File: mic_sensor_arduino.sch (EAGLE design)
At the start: 19 parts, among them U1 LM393DR, U2 LM393DR

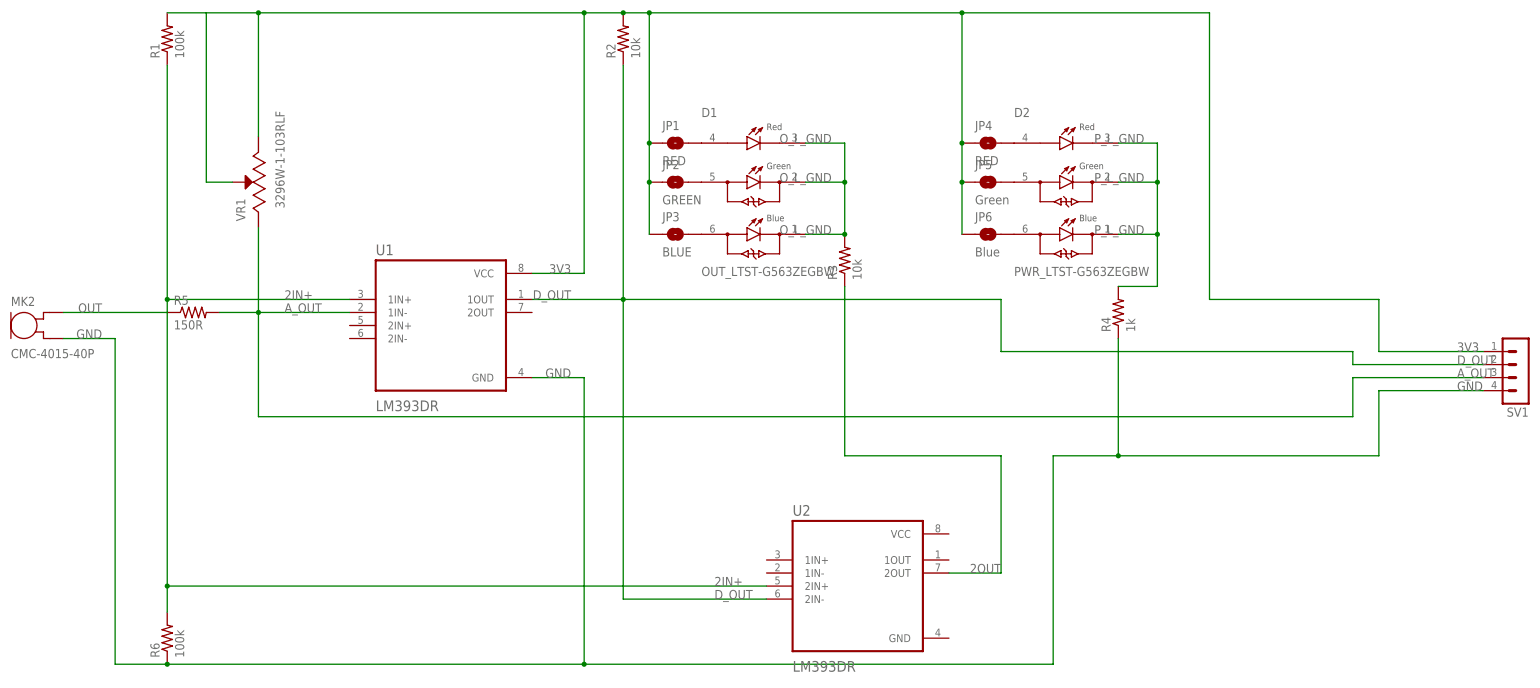
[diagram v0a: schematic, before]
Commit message: update resources
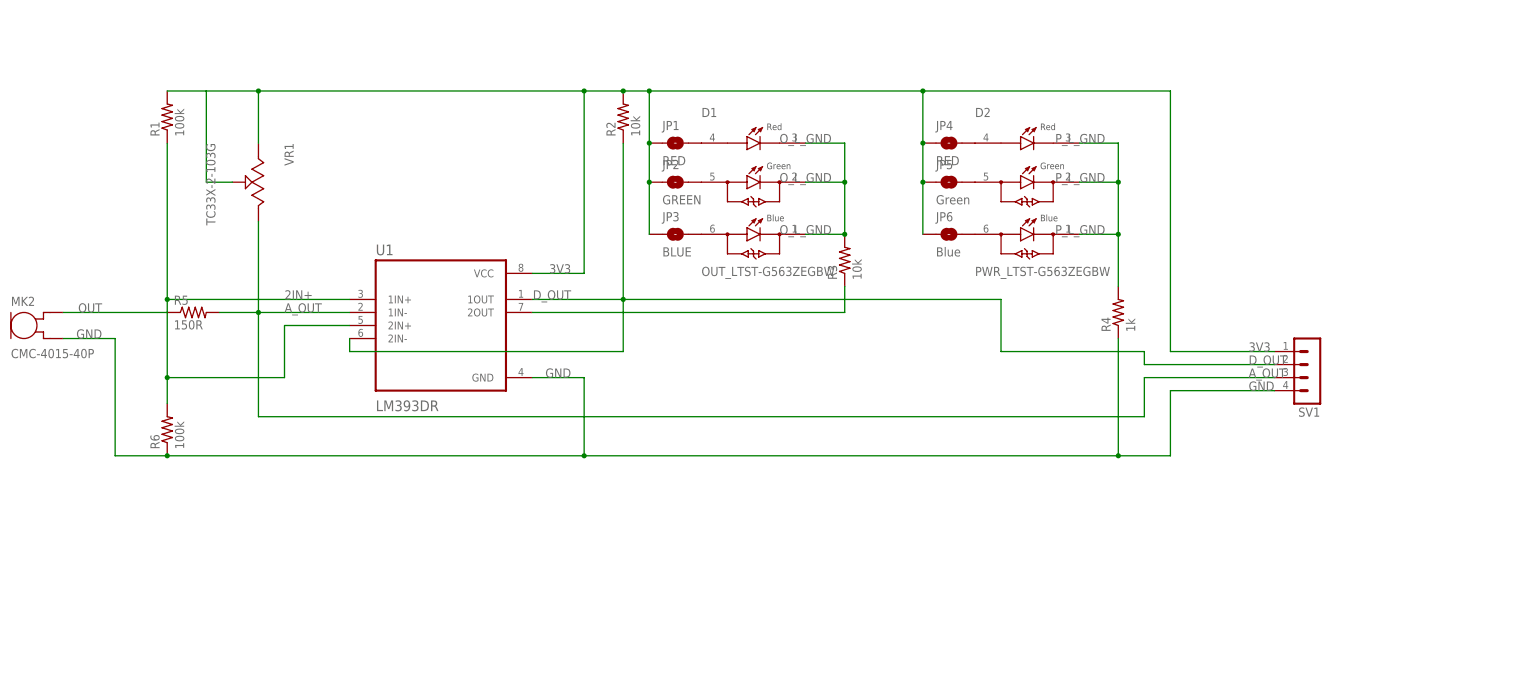
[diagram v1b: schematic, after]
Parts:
- removed U2: LM393DR, LM393DR:LM393DR
- VR1: value 3296W-1-103RLF -> TC33X-2-103G; device 3296W-1-103RLF:3296W-1-103RLF -> TC33X-2-103G:TC33X-2-103G
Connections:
- net 2IN+: now also U1.2IN+; no longer U2.2IN+
- net 2OUT: now also U1.2OUT; no longer U2.2OUT
- net 3V3: now also VR1.CCW; no longer VR1.CW
- net A_OUT: now also VR1.CW; no longer VR1.CCW
- net D_OUT: now also U1.2IN-; no longer U2.2IN-
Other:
- moved on the sheet: D2, JP4, JP5, JP6, R1, R2, R6, SV1
